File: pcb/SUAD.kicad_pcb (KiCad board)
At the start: 2 copper layers, 100 x 102.5 mm, 89 parts, among them Q1 AO3401A, Q2 AO3401A, Q3 AO3401A, SW1 SW_MEC_5E, SW10 SW_MEC_5E, SW11 SW_MEC_5E, SW12 SW_MEC_5E, SW13 SW_DIP_x06, SW2 SW_MEC_5E, SW3 SW_MEC_5E, SW4 SW_MEC_5E, SW5 SW_MEC_5E, SW6 SW_MEC_5E, SW7 SW_MEC_5E, SW8 SW_MEC_5E, SW9 SW_MEC_5E, U1 Pico

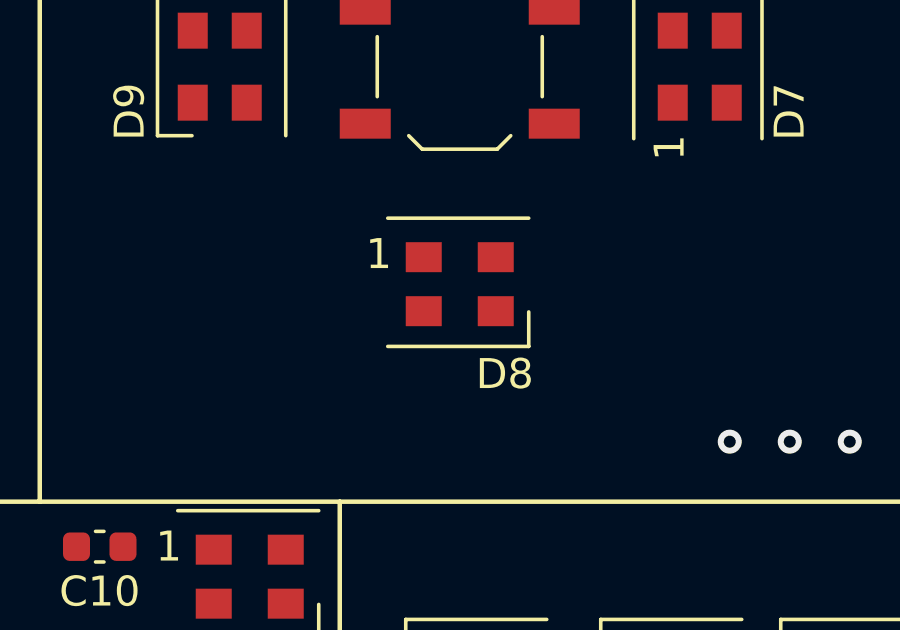
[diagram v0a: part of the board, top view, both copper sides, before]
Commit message: workflow trigger
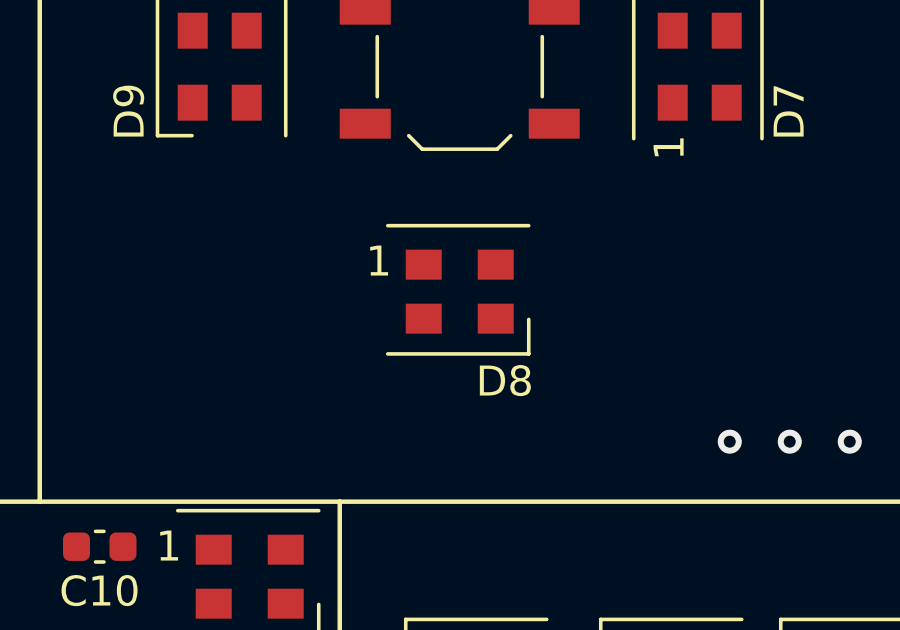
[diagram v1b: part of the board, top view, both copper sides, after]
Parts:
- moved D8 0.25 mm to (160.0, 115.0)
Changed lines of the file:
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@@
   )
   (footprint "LCSC_parts:LED_WS2812B-Mini_3.5x3.5mm" (layer "F.Cu")
-    (at 160 114.75)
+    (at 160 115)
     (descr "https://datasheet.lcsc.com/lcsc/2005251033_Worldsemi-WS2812B-Mini_C527089.pdf")
     (tags "LED RGB")

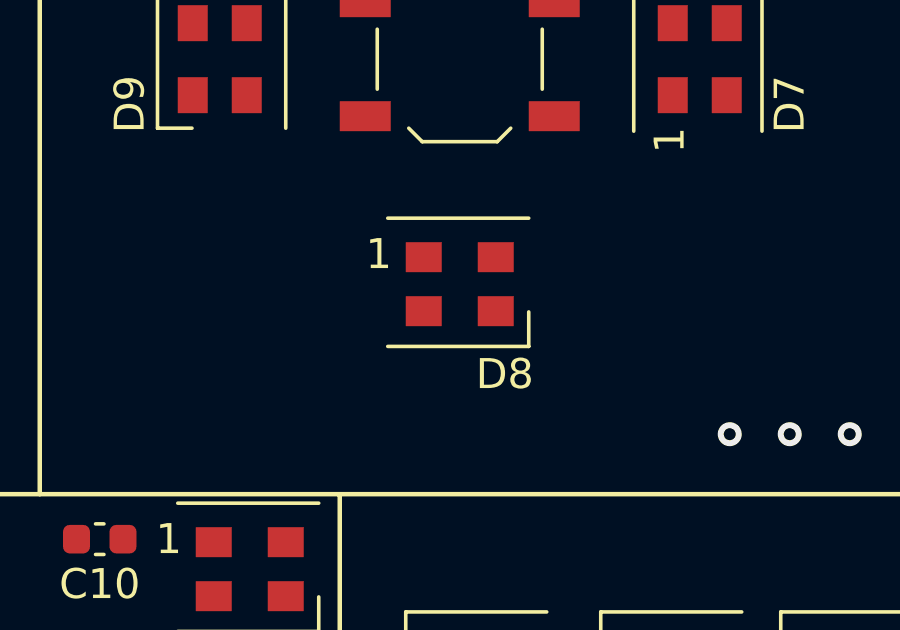
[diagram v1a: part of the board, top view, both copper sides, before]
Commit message: workflow trigger
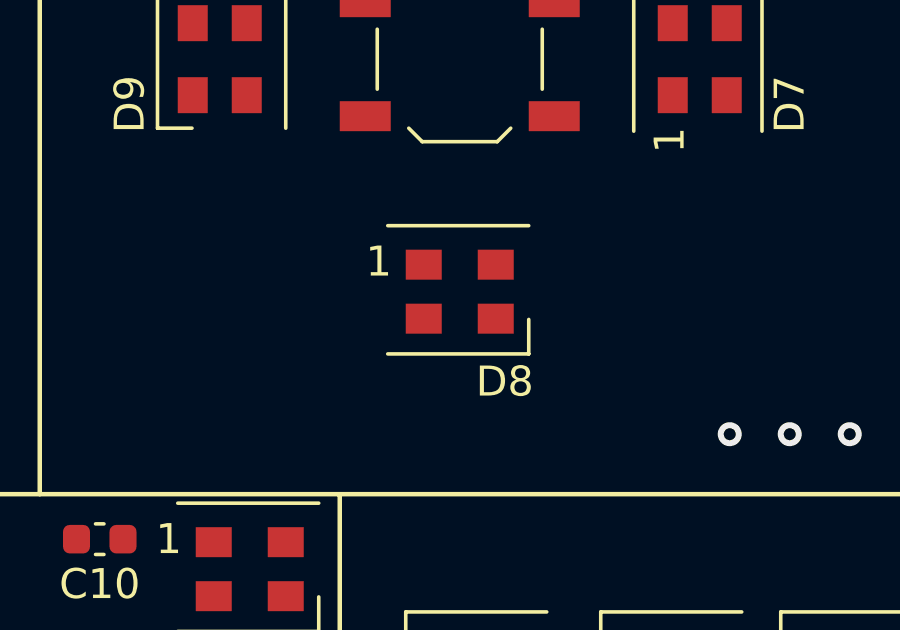
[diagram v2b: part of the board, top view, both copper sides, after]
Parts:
- moved D8 0.25 mm to (160.0, 115.2)
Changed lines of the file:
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@@
   )
   (footprint "LCSC_parts:LED_WS2812B-Mini_3.5x3.5mm" (layer "F.Cu")
-    (at 160 115)
+    (at 160 115.25)
     (descr "https://datasheet.lcsc.com/lcsc/2005251033_Worldsemi-WS2812B-Mini_C527089.pdf")
     (tags "LED RGB")

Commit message: workflow trigger
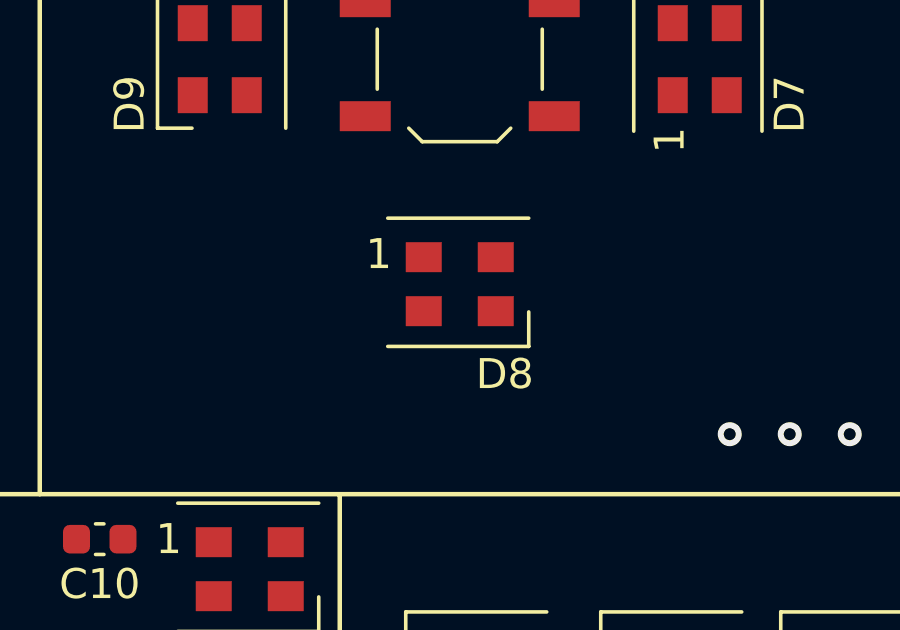
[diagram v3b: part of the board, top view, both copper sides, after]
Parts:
- moved D8 0.25 mm to (160.0, 115.0)
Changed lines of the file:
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@@
   )
   (footprint "LCSC_parts:LED_WS2812B-Mini_3.5x3.5mm" (layer "F.Cu")
-    (at 160 115.25)
+    (at 160 115)
     (descr "https://datasheet.lcsc.com/lcsc/2005251033_Worldsemi-WS2812B-Mini_C527089.pdf")
     (tags "LED RGB")

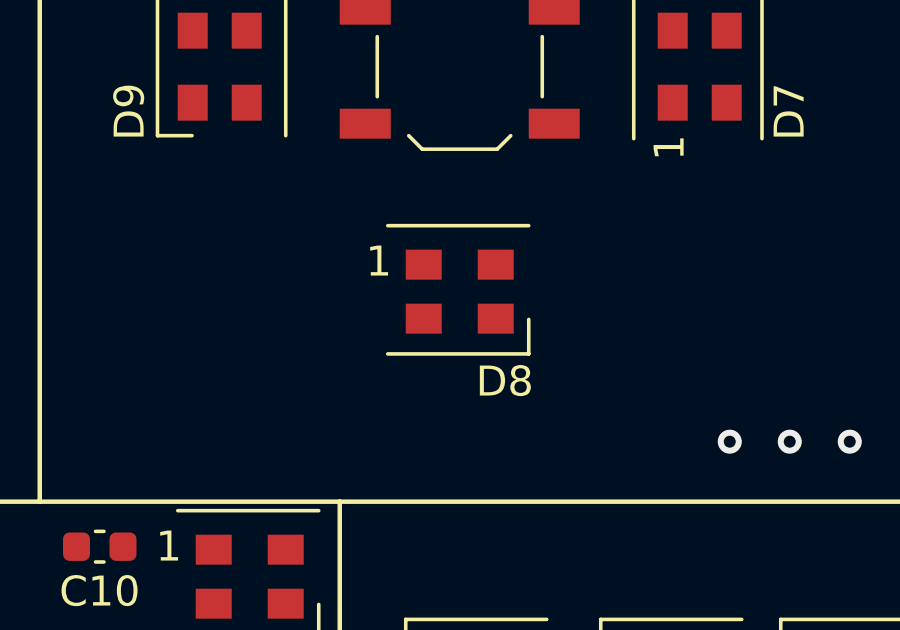
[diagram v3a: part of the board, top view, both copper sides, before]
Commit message: workflow trigger
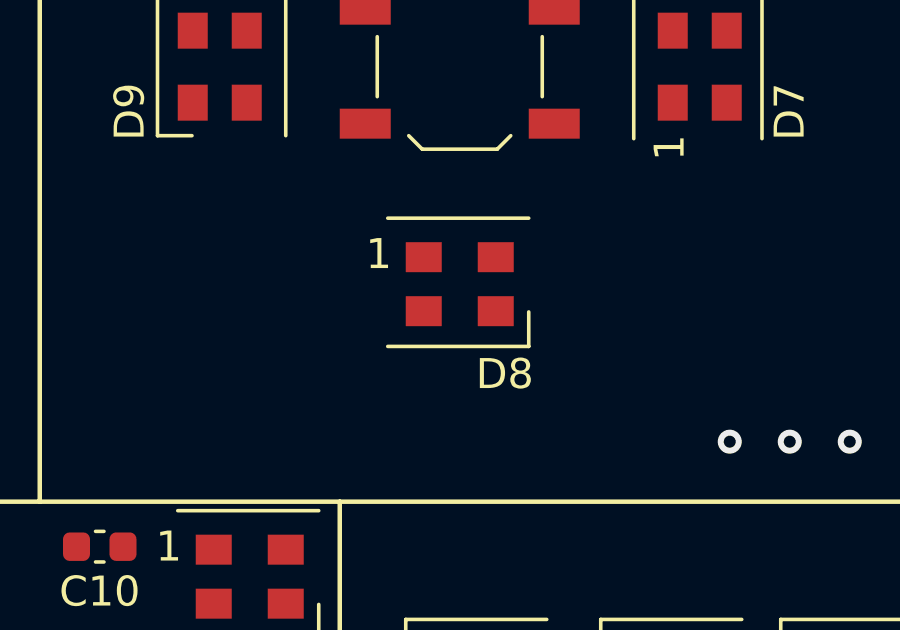
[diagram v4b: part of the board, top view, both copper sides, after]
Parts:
- moved D8 0.25 mm to (160.0, 114.8)
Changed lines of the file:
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@@
   )
   (footprint "LCSC_parts:LED_WS2812B-Mini_3.5x3.5mm" (layer "F.Cu")
-    (at 160 115)
+    (at 160 114.75)
     (descr "https://datasheet.lcsc.com/lcsc/2005251033_Worldsemi-WS2812B-Mini_C527089.pdf")
     (tags "LED RGB")
